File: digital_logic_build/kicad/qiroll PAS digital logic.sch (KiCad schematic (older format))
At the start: 47 parts, among them J2 led_sw1, J3 accessory, J4 mode_thr_batt, J5 3_pin, U1 4093B, U2 4027B, U3 4093B, U5 4093B, U6 14538B, U7 MCP1799_3V3

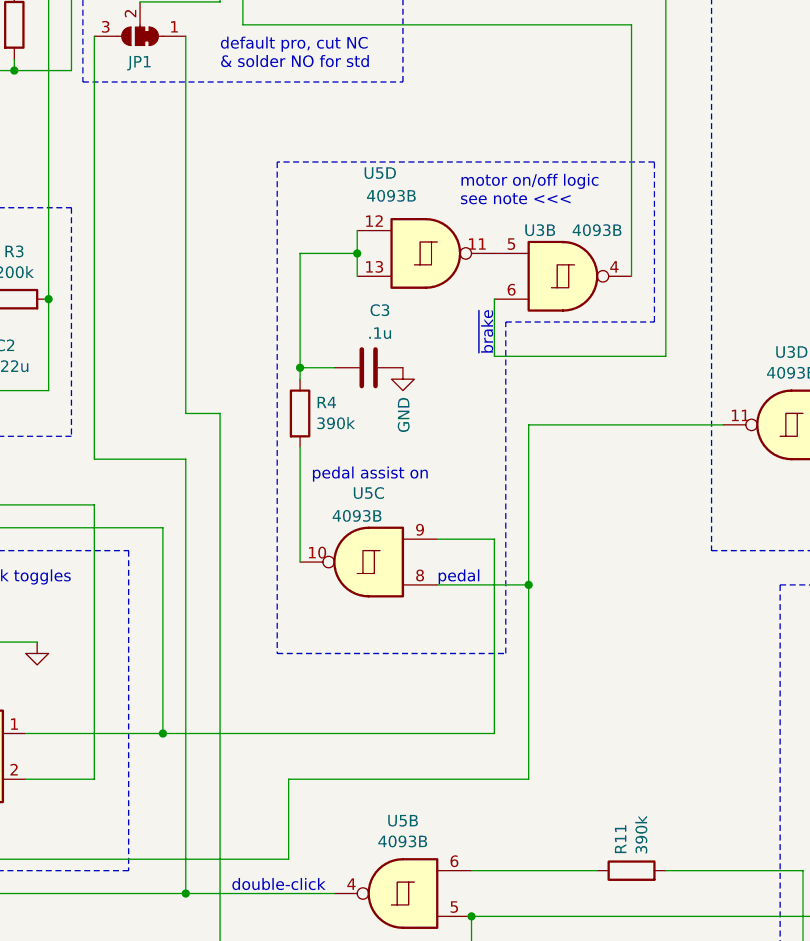
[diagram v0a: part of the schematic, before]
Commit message: even tidier schematic
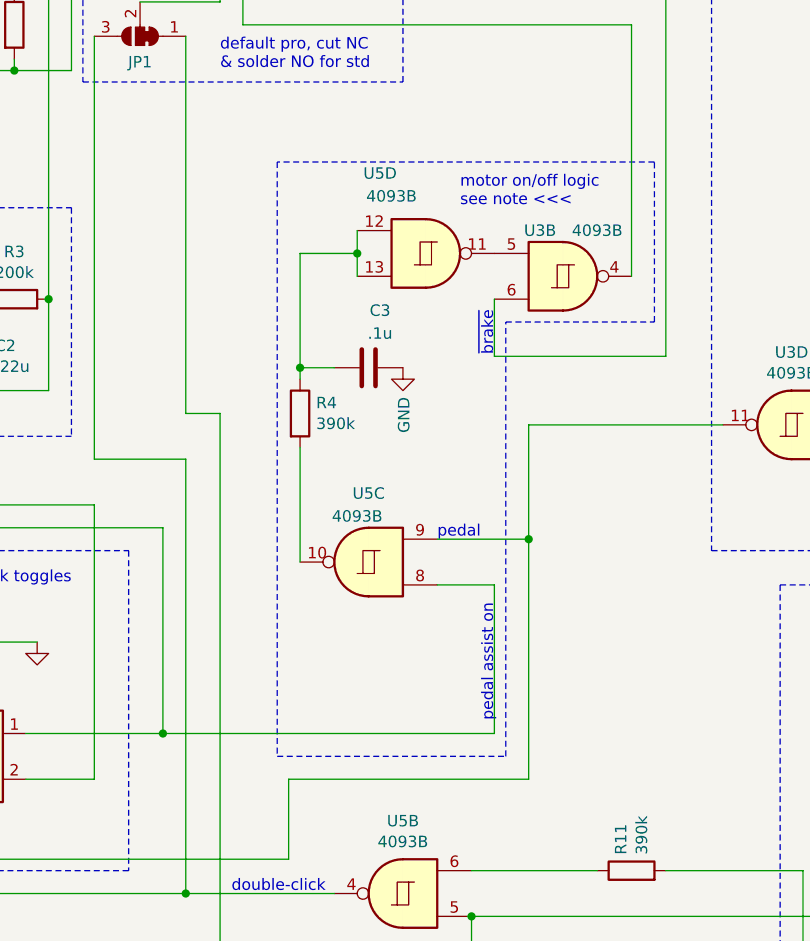
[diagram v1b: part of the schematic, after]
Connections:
- net at U1.9, U2.1 (Q): now also U5.8; no longer U5.9
- net at U2.12 (R), U3.11: now also U5.9; no longer U5.8
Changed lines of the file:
@@
 Text Notes 550  1950 0    50   Italic 0
 note: pedal cadence sense\ncadence threshold is nominally\n40rpm on/29rpm off, \nwith C6 installed, C5 uninstalled,\nand typical 4093 Vp/Vn values\n(Vp = 3.3, Vn = 2.3)\n\ninstall C5+C6 to lower threshold, or\nmake up for 4093 Vp/Vn variation\n\ninstall C5 only to raise threshold, or\nmake up for 4093 Vp/Vn variation\n
-Text Notes 6900 4650 0    50   ~ 0
+Text Notes 6900 4450 0    50   ~ 0
 pedal
-Text Notes 6350 4200 0    50   ~ 0
+Text Notes 7150 5250 1    50   ~ 0
 pedal assist on
 $Comp
@@
 	2000 600  5000 600
 Wire Notes Line
-	6200 2800 6200 4950
-Wire Notes Line
-	6200 4950 7200 4950
-Wire Notes Line
-	7200 4950 7200 3500
+	6200 2800 6200 5400
+Wire Notes Line
+	6200 5400 7200 5400
+Wire Notes Line
+	7200 5400 7200 3500
 Wire Notes Line
 	7200 3500 7850 3500
@@
 Connection ~ 9050 3400
 Wire Wire Line
-	7300 4650 7300 5500
+	7300 4450 7300 5500
 Connection ~ 8850 4050
 Wire Wire Line
@@
 	2250 2200 2250 4250
 Wire Wire Line
-	7300 4650 6900 4650
+	7300 4450 6900 4450
 Wire Wire Line
 	6300 4050 6300 4550
@@
 $EndComp
 Wire Wire Line
-	7150 5300 7150 4450
-Wire Wire Line
-	7150 4450 6900 4450
-Wire Wire Line
 	5700 5300 7150 5300
 Wire Notes Line
@@
 	8150 3950 7300 3950
 Wire Wire Line
-	7300 3950 7300 4650
-Connection ~ 7300 4650
+	7300 3950 7300 4450
+Connection ~ 7300 4450
 Wire Notes Line
 	5350 2450 6750 2450
@@
 	9000 2600 9000 2550
 $Comp
-L power:VDD #PWR?
+L power:VDD #PWR0104
 U 1 1 622AB00C
 P 9050 3100
-F 0 "#PWR?" H 9050 2950 50  0001 C CNN
+F 0 "#PWR0104" H 9050 2950 50  0001 C CNN
 F 1 "VDD" H 9065 3273 50  0000 C CNN
 F 2 "" H 9050 3100 50  0001 C CNN
@@
 Text Notes 2200 2800 1    50   ~ 0
 install\nD5 for Pro kit only
+Wire Wire Line
+	7150 4650 6900 4650
+Wire Wire Line
+	7150 4650 7150 5300
 $EndSCHEMATC
